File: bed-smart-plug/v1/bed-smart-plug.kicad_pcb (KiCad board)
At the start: 2 copper layers, 122.6 x 80.6 mm, 26 parts, among them J1 DS18b20, J2 Conn_01x02_Male, J3 3.5mm headphone jack, J4 Triac gate protection, J5 Opto snubber, J6 Opto snubber 2, J7 Main, J8 Triac snubber, J9 Prises, Q1 BT136-600E, U1 ESP32-POE, U2 AM-RX12A-433P, U3 MOC3021M

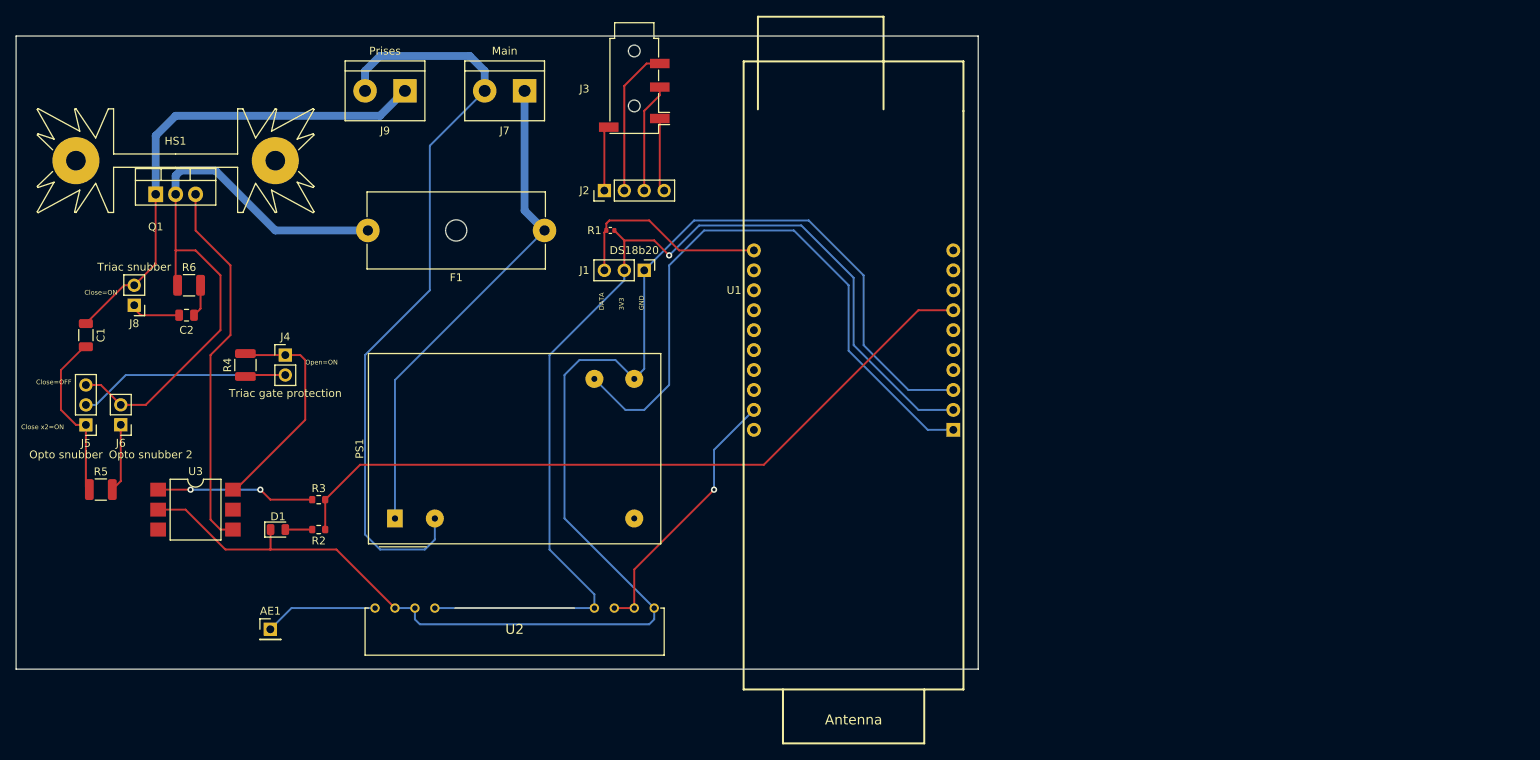
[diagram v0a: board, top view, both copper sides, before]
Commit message: wip pcb v1
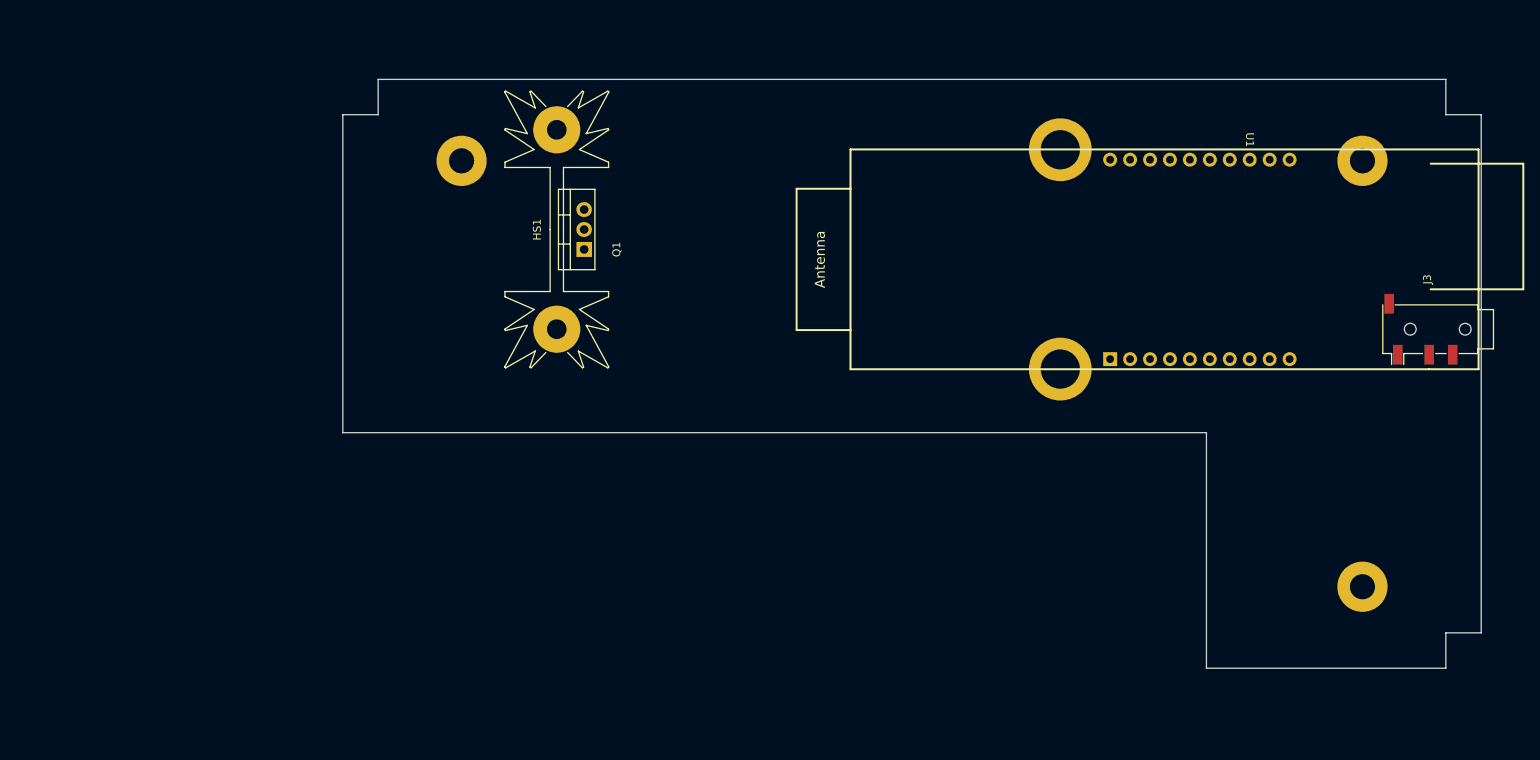
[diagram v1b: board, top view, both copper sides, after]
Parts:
- removed AE1: Antenna, Connector_PinHeader_2.54mm:PinHeader_1x01_P2.54mm_Vertical
- removed C1: 47nF/400V, Capacitor_SMD:C_1206_3216Metric
- removed C2: 10nF/400V, Capacitor_SMD:C_0805_2012Metric
- removed D1: LED, Diode_SMD:D_0805_2012Metric
- removed F1: 3A, Fuse:Fuseholder_Cylinder-5x20mm_Schurter_0031_8201_Horizontal_Open
- removed J1: DS18b20, Connector_PinHeader_2.54mm:PinHeader_1x03_P2.54mm_Vertical
- removed J2: Conn_01x02_Male, Connector_PinHeader_2.54mm:PinHeader_1x04_P2.54mm_Vertical
- removed J4: Triac gate protection, Connector_PinHeader_2.54mm:PinHeader_1x02_P2.54mm_Vertical
- removed J5: Opto snubber, Connector_PinHeader_2.54mm:PinHeader_1x03_P2.54mm_Vertical
- removed J6: Opto snubber 2, Connector_PinHeader_2.54mm:PinHeader_1x02_P2.54mm_Vertical
- removed J7: Main, TerminalBlock:TerminalBlock_bornier-2_P5.08mm
- removed J8: Triac snubber, Connector_PinHeader_2.54mm:PinHeader_1x02_P2.54mm_Vertical
- removed J9: Prises, TerminalBlock:TerminalBlock_bornier-2_P5.08mm
- removed PS1: Alim RS PRO 5V 1A, Converter_ACDC:Converter_ACDC_MeanWell_IRM-03-xx_THT
- removed R1: 4.7KΩ, Resistor_SMD:R_0402_1005Metric
- removed R2, R3: 220Ω, Resistor_SMD:R_0603_1608Metric
- removed R4: 360Ω/0.5W, Resistor_SMD:R_1210_3225Metric
- removed R5: 470Ω/0.5W, Resistor_SMD:R_1210_3225Metric
- removed R6: 39Ω/0.5W, Resistor_SMD:R_1210_3225Metric
- removed U2: AM-RX12A-433P, mylife-footprints:AMRX12A433P
- removed U3: MOC3021M, Package_DIP:SMDIP-6_W9.53mm
- added ?: , , F.Cu at (202.0, 57.2)
- added ?: , , F.Cu at (163.5, 83.7)
- added ?: , , F.Cu at (87.2, 57.2)
- added ?: , , F.Cu at (163.5, 55.8)
- added ?: , , F.Cu at (202.0, 111.4)
- moved J3 105.6 mm to (210.3, 78.6), turned to 180 degrees
- moved Q1 55.0 mm to (102.8, 68.5), turned to 90 degrees
- moved HS1 49.3 mm to (99.3, 65.9), turned to 90 degrees
- moved U1 44.3 mm to (179.9, 69.7), turned to 90 degrees
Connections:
- Q1 pad 1: Net-(J8-Pin_2) -> (no net)
- Q1 pad 2: Net-(J5-Pin_3) -> (no net)
- Q1 pad 3: Net-(Q1-G) -> (no net)
- U1 pad 1: +5V -> (no net)
- U1 pad 11: Net-(J1-Pin_3) -> (no net)
- U1 pad 19: Net-(U1-GPIO36) -> (no net)
- U1 pad 2: +3V3 -> (no net)
- U1 pad 3: GND -> (no net)
- U1 pad 7: Net-(U1-GPIO2) -> (no net)
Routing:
- net GND: track 189.9 -> 0.00 mm
- net +3V3: track 134.3 -> 0.00 mm, vias 1 -> 0
- net NEUT: track 97.6 -> 0.00 mm
- net Net-(U1-GPIO2): track 93.8 -> 0.00 mm
- net +5V: track 81.2 -> 0.00 mm
- net Net-(J5-Pin_3): track 78.1 -> 0.00 mm
- net LINE: track 63.4 -> 0.00 mm
- net Net-(J8-Pin_2): track 62.5 -> 0.00 mm
- net Net-(Q1-G): track 47.7 -> 0.00 mm
- net Net-(U1-GPIO36): track 34.1 -> 0.00 mm, vias 1 -> 0
- net Net-(J4-Pin_2): track 32.1 -> 0.00 mm
- net Net-(J4-Pin_1): track 28.5 -> 0.00 mm
- net Net-(J1-Pin_3): track 26.6 -> 0.00 mm
- net Net-(J5-Pin_1): track 21.9 -> 0.00 mm
- net Net-(R3-Pad1): track 20.2 -> 0.00 mm, vias 2 -> 0
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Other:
- board size 122.6 x 80.6 mm -> 145 x 75 mm
- board text removed: "3V3"
- board text removed: "Close x2=ON"
- board text removed: "Close=OFF"
- board text removed: "Close=ON"
- board text removed: "DATA"
- board text removed: "GND"
- board text removed: "Open=ON"
